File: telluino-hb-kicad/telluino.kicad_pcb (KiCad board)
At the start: 2 copper layers, 90 x 38 mm, 74 parts, among them J1 6P2C, J2 USB_A, Q1 MMBT3904, U1 LE9641PQC, U2 TISP61089BDR-S, U3 CH340C, U4 TXS0108EPWRG4

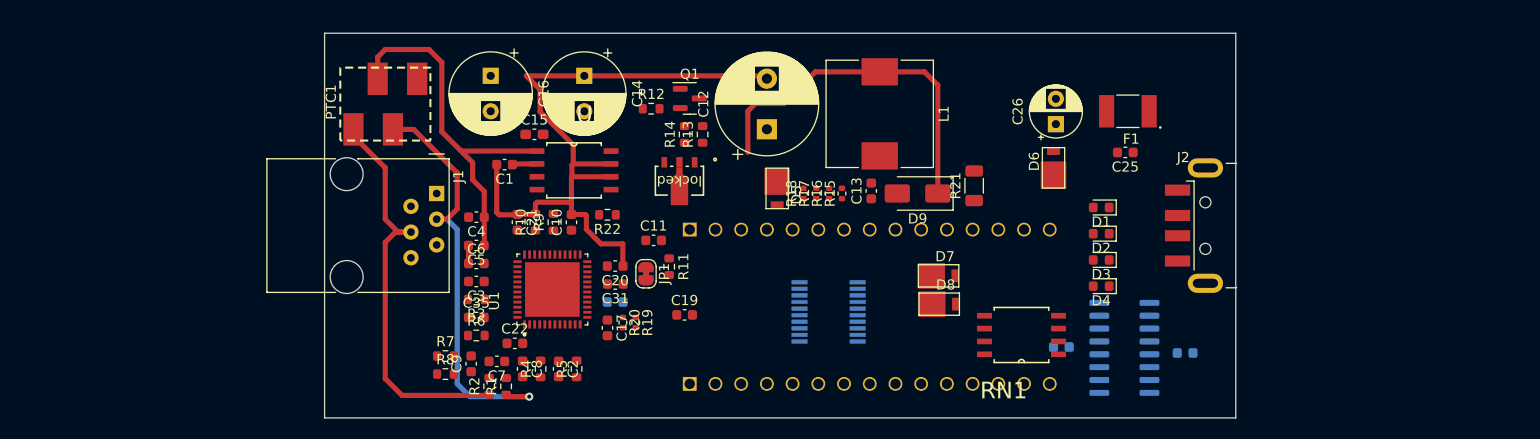
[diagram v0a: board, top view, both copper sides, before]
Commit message: placement done
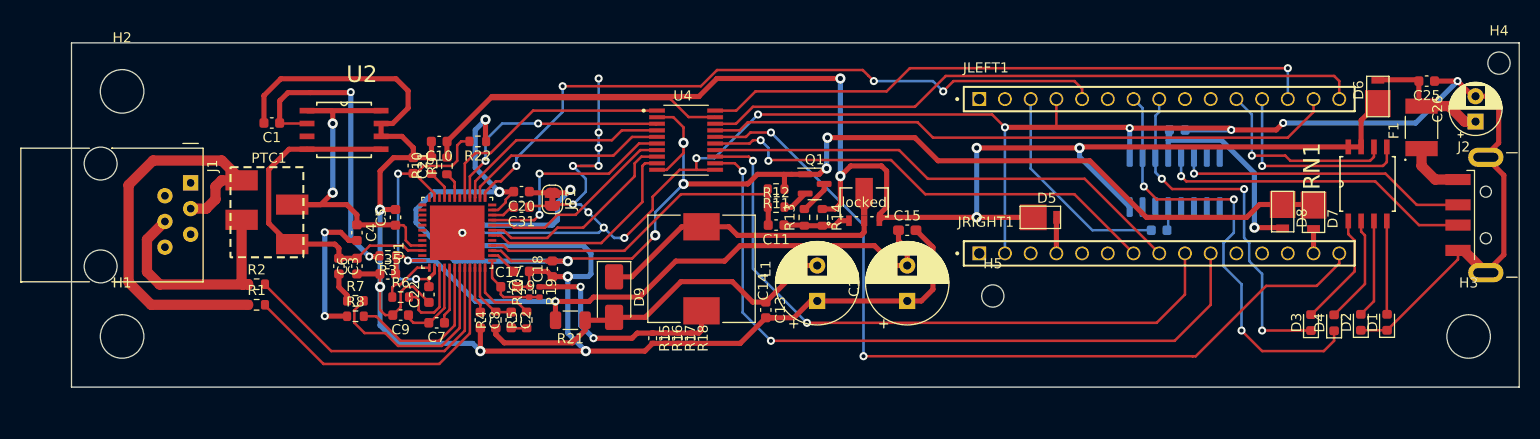
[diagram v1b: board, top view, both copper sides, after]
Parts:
- removed C12: 220uF/25V, Capacitor_THT:CP_Radial_D10.0mm_P5.00mm
- added H1: MountingHole, MountingHole:MountingHole_4.3mm_M4, F.Cu at (76.3, 107.0)
- added H2: MountingHole, MountingHole:MountingHole_4.3mm_M4, F.Cu at (76.3, 82.7)
- added H3: MountingHole, MountingHole:MountingHole_4.3mm_M4, F.Cu at (209.3, 107.0)
- added H4: MountingHole, MountingHole:MountingHole_2.2mm_M2, F.Cu at (212.3, 80.0)
- added H5: MountingHole, MountingHole:MountingHole_2.2mm_M2, F.Cu at (162.3, 103.0)
- C18, JLEFT1, JRIGHT1, U4: moved to F.Cu
- moved C16 46.8 mm to (153.8, 103.4), turned to 90 degrees
- moved R21 42.0 mm to (120.5, 105.3), turned to 180 degrees
- moved C26 41.5 mm to (209.9, 85.7)
- moved JLEFT1 40.1 mm to (178.7, 83.5)
- moved C15 38.0 mm to (153.8, 96.5)
- moved D7 37.6 mm to (193.9, 94.7), turned to -90 degrees
- moved RN1 37.3 mm to (199.3, 91.9), turned to 90 degrees
- moved D8 35.1 mm to (190.9, 94.6), turned to -90 degrees
- moved D6 32.8 mm to (200.3, 83.2)
- moved C14 32.0 mm to (144.9, 103.4), turned to 90 degrees
- moved D9 31.7 mm to (124.9, 103.1), turned to -90 degrees
- moved C25 30.6 mm to (205.1, 81.7)
- moved D1 30.4 mm to (201.2, 105.6), turned to 90 degrees
- moved F1 29.0 mm to (204.6, 86.3), turned to 90 degrees
- moved JRIGHT1 28.7 mm to (178.7, 98.7)
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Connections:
- net Net-(U1A-RINGD1) renamed /RING
- net Net-(U1A-TIPD1) renamed /TIP
- J1 pad 3: Net-(J1-Pad3) -> /RING_IN
- J1 pad 4: Net-(J1-Pad4) -> /TIP_IN
- JLEFT1 pad 07: USB_RX1 -> USB_TX1
- JLEFT1 pad 08: USB_TX1 -> USB_RX1
- JLEFT1 pad 11: OP1_LED -> OP2_LED
- JLEFT1 pad 12: OP2_LED -> OP1_LED
- PTC1 pad 1: Net-(J1-Pad4) -> /RING_IN
- PTC1 pad 3: Net-(J1-Pad3) -> /TIP_IN
- R1 pad 1: Net-(J1-Pad3) -> /RING_IN
- R2 pad 1: Net-(J1-Pad4) -> /TIP_IN
- RN1 pad 1: Net-(D4-A) -> Net-(D3-A)
- RN1 pad 2: Net-(D3-A) -> Net-(D4-A)
- U4 pad 1: DCLK -> CS_N
- U4 pad 12: PCLK_5 -> FS_5
- U4 pad 13: DRA_5 -> DXA_5
- U4 pad 14: DXA_5 -> DRA_5
- U4 pad 15: FS_5 -> PCLK_5
- U4 pad 16: DOUT_5 -> DCLK_5
- U4 pad 18: CS_N_5 -> DOUT_5
- U4 pad 20: DCLK_5 -> CS_N_5
- U4 pad 3: CS_N -> DOUT
- U4 pad 5: DOUT -> DCLK
- U4 pad 6: FS -> PCLK
- U4 pad 7: DXA -> DRA
- U4 pad 8: DRA -> DXA
- U4 pad 9: PCLK -> FS
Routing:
- net GNDD: track 0.00 -> 208.1 mm, vias 0 -> 17
- net +5V: track 0.00 -> 170.0 mm, vias 0 -> 5
- net +3.3V: track 0.00 -> 153.9 mm, vias 0 -> 8
- net GNDA: track 71.5 -> 191.8 mm, vias 0 -> 6
- net DCLK_5: track 0.00 -> 83.4 mm, vias 0 -> 2
- net FS_5: track 0.00 -> 70.9 mm, vias 0 -> 2
- net INT_N: track 0.00 -> 69.4 mm, vias 0 -> 4
- net VBAT: track 0.00 -> 65.8 mm, vias 0 -> 2
- net DOUT_5: track 0.00 -> 65.6 mm
- net DXA_5: track 0.00 -> 64.7 mm, vias 0 -> 2
- net DIN_5: track 0.00 -> 62.4 mm
- net CS_N_5: track 0.00 -> 61.3 mm, vias 0 -> 1
- net DRA_5: track 0.00 -> 48.1 mm
- net PCLK_5: track 0.00 -> 46.9 mm, vias 0 -> 2
- net USB_TX1: track 0.00 -> 43.9 mm, vias 0 -> 3
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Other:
- board size 90 x 38 mm -> 143 x 34 mm
